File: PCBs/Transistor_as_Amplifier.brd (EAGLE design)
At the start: 37.5 x 25.9 mm, 12 parts, among them T1 BC547N

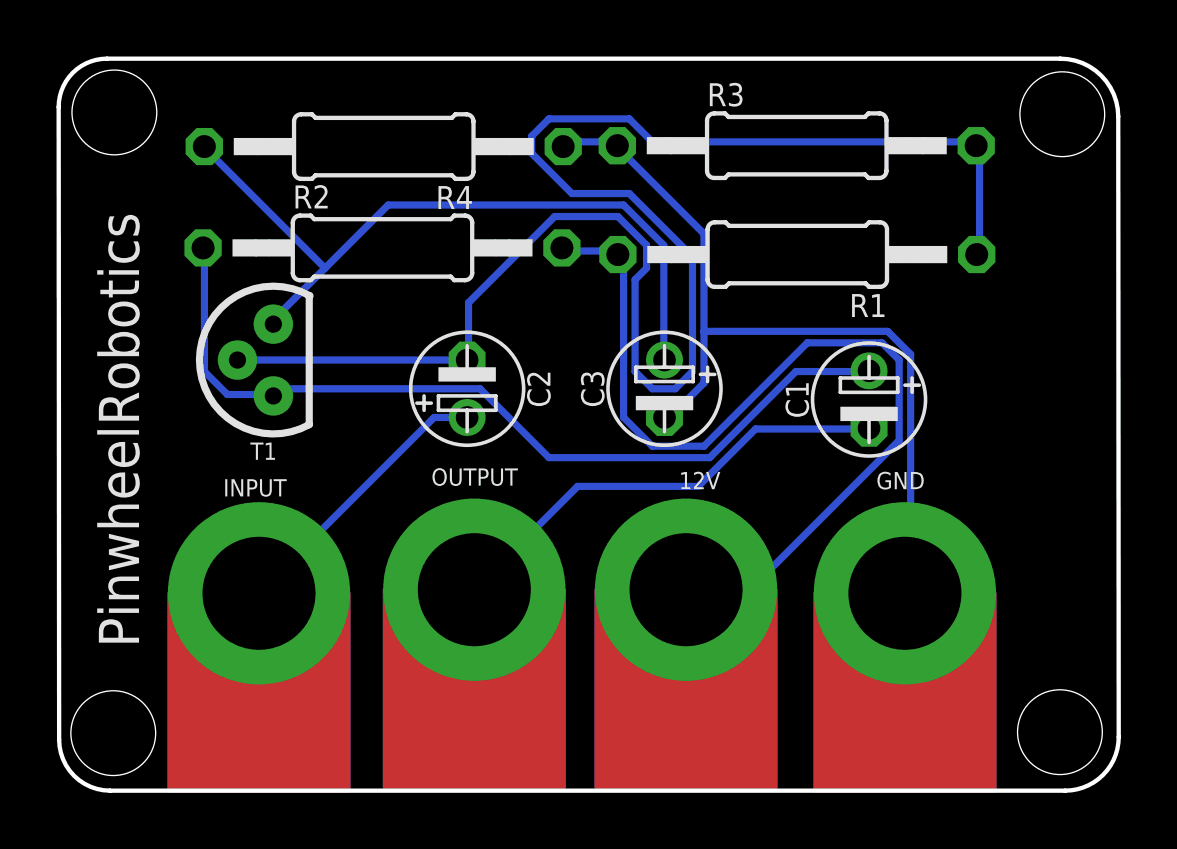
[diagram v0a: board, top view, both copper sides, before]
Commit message: New Update
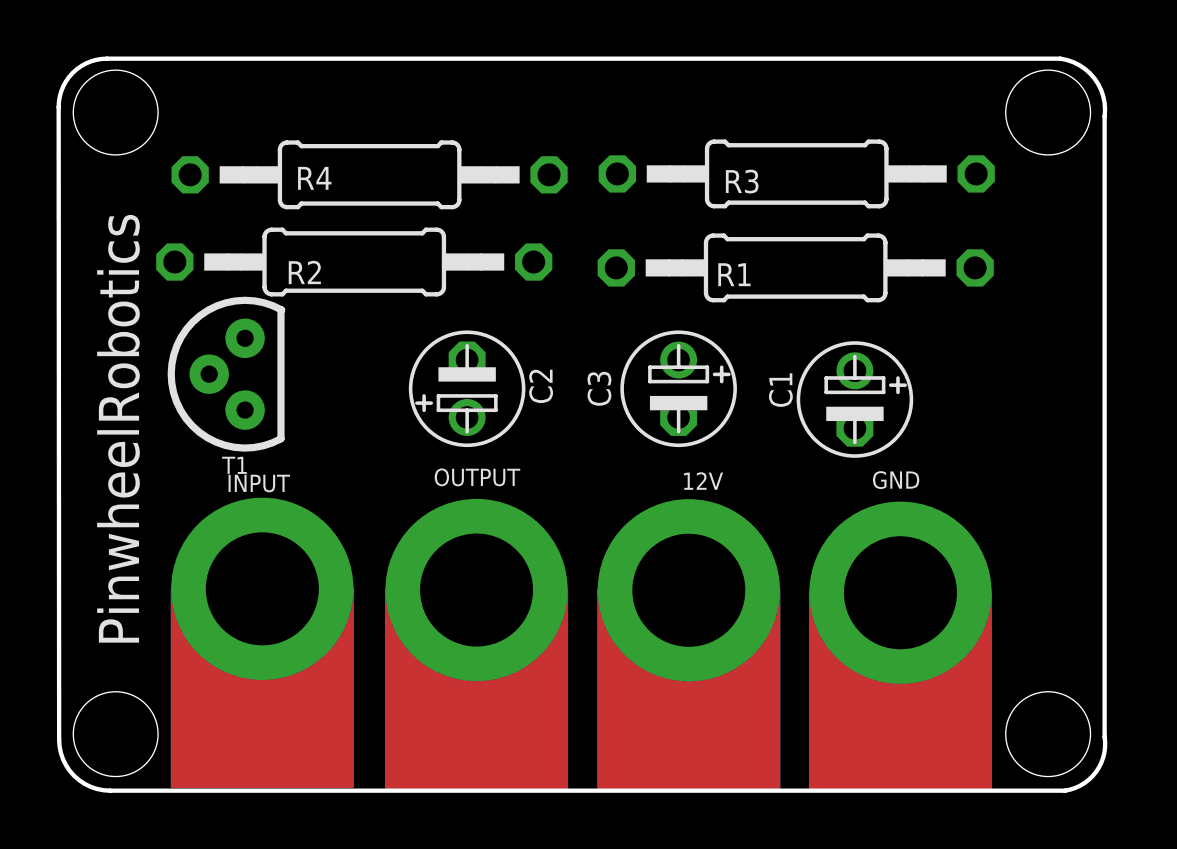
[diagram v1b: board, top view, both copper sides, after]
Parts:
- moved R2 1.12 mm to (7.94, 18.7)
- moved R4 1.12 mm to (8.49, 21.8)
- moved T1 1.12 mm to (4.08, 13.5)
- moved R3 1.00 mm to (23.6, 21.8)
- moved C1 0.50 mm to (25.7, 13.8)
- moved C3 0.50 mm to (19.4, 14.2)
- moved R1 0.47 mm to (23.6, 18.5)
- moved INPUT 0.20 mm to (4.69, 7.14)
- moved GND 0.16 mm to (27.3, 7.00)
- moved 12V 0.10 mm to (19.8, 7.09)
- moved OUTPUT 0.08 mm to (12.3, 7.10)
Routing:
- net N$3: track 57.6 -> 0.00 mm
- net 12V: track 32.6 -> 0.00 mm
- net N$2: track 30.7 -> 0.00 mm
- net GND: track 29.8 -> 0.00 mm
- net N$1: track 26.4 -> 0.00 mm
- net N$4: track 16.3 -> 0.00 mm
- net N$7: track 9.95 -> 0.00 mm
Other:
- board size 37.5 x 25.9 mm -> 37 x 25.9 mm
